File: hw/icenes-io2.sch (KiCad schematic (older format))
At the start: 35 parts, among them J4 Conn_02x31_Odd_Even, J5 Conn_02x31_Odd_Even, U4 iCE40HX8K-CT256, X2 DSC1001BI2-133.0000T

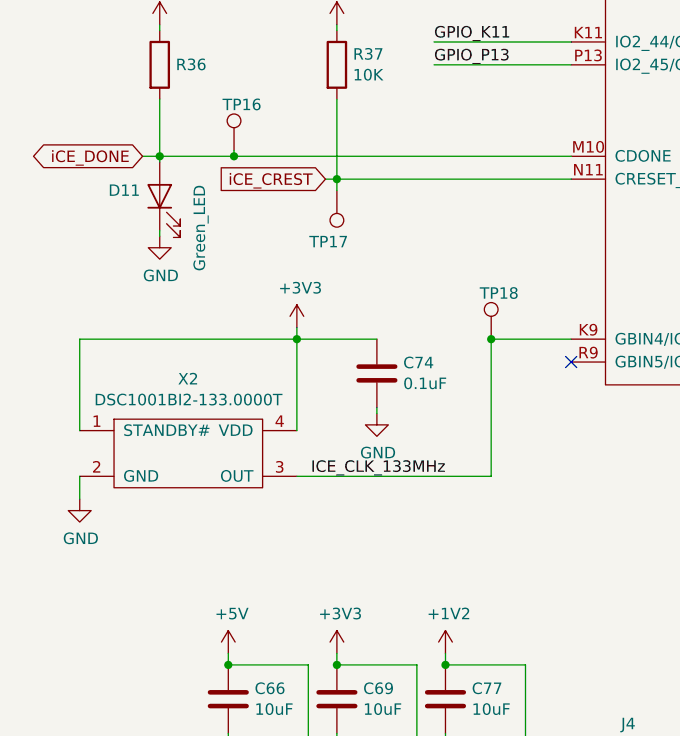
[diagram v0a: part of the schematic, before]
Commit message: Rough board layout.
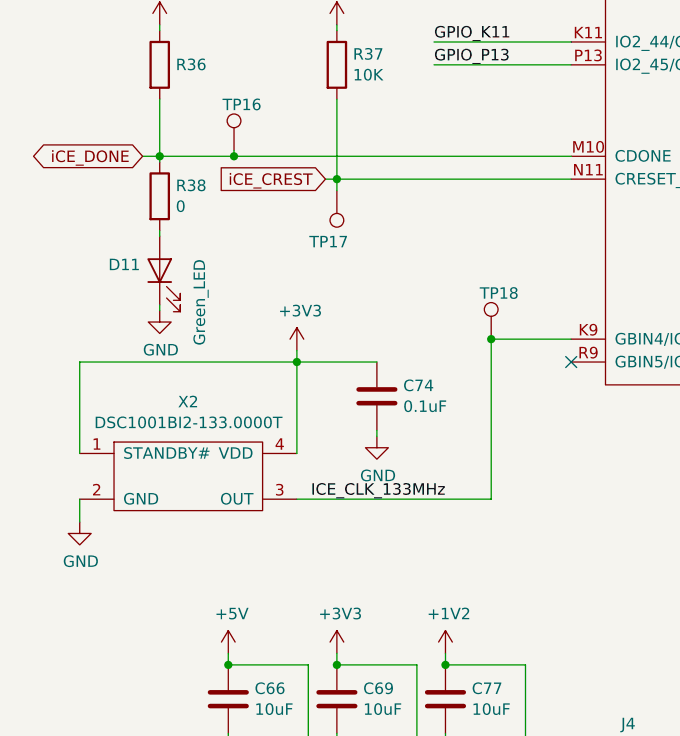
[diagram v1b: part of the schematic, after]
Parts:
- added R38: R0_0603, Resistor_SMD:R_0603_1608Metric_Pad1.05x0.95mm_HandSolder, symbol icenes-library:R0_0603
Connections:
- net iCE_DONE: now also R38.1; no longer D11.2 (A)
- new net: D11.2 (A), R38.2
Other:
- moved on the sheet: C74, D11, X2
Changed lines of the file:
@@
 L icenes-library:Green_LED D11
 U 1 1 5DA2730F
-P 1300 4775
-F 0 "D11" V 1325 5000 50  0000 R CNN
-F 1 "Green_LED" H 1350 4600 50  0000 R CNN
-F 2 "LED_SMD:LED_0805_2012Metric_Pad1.15x1.40mm_HandSolder" H 1300 4775 50  0001 C CNN
-F 3 "https://www.mouser.se/datasheet/2/216/APTD2012LCGCK-1102037.pdf" H 1300 4775 50  0001 C CNN
-F 4 "Kingbright" H 1300 4775 50  0001 C CNN "Manufacturer"
-F 5 "APTD2012LCGCK" H 1300 4775 50  0001 C CNN "Part number"
-	1    1300 4775
+P 1300 5100
+F 0 "D11" V 1325 5325 50  0000 R CNN
+F 1 "Green_LED" H 1350 4925 50  0000 R CNN
+F 2 "LED_SMD:LED_0805_2012Metric_Pad1.15x1.40mm_HandSolder" H 1300 5100 50  0001 C CNN
+F 3 "https://www.mouser.se/datasheet/2/216/APTD2012LCGCK-1102037.pdf" H 1300 5100 50  0001 C CNN
+F 4 "Kingbright" H 1300 5100 50  0001 C CNN "Manufacturer"
+F 5 "APTD2012LCGCK" H 1300 5100 50  0001 C CNN "Part number"
+	1    1300 5100
 	0    -1   -1   0
 $EndComp
@@
 L power:GND #PWR?
 U 1 1 5DA5244F
-P 1300 4950
+P 1300 5275
 AR Path="/5D1BB1FB/5DA5244F" Ref="#PWR?"  Part="1"
 AR Path="/5D1BB49B/5DA5244F" Ref="#PWR090"  Part="1"
-F 0 "#PWR090" H 1300 4700 50  0001 C CNN
-F 1 "GND" H 1305 4777 50  0000 C CNN
-F 2 "" H 1300 4950 50  0001 C CNN
-F 3 "" H 1300 4950 50  0001 C CNN
-	1    1300 4950
+F 0 "#PWR090" H 1300 5025 50  0001 C CNN
+F 1 "GND" H 1305 5102 50  0000 C CNN
+F 2 "" H 1300 5275 50  0001 C CNN
+F 3 "" H 1300 5275 50  0001 C CNN
+	1    1300 5275
 	1    0    0    -1
 $EndComp
@@
 	1300 4025 1300 4050
 Wire Wire Line
-	1300 4925 1300 4950
+	1300 5250 1300 5275
 Wire Wire Line
 	1225 4600 1300 4600
@@
 L icenes-library:C0.1uF C?
 U 1 1 5DC56E81
-P 2250 5550
+P 2250 5650
 AR Path="/5D1BAC88/5DC56E81" Ref="C?"  Part="1"
 AR Path="/5D1BB49B/5DC56E81" Ref="C74"  Part="1"
-F 0 "C74" H 2365 5596 50  0000 L CNN
-F 1 "C0.1uF" H 2100 5450 50  0001 C CNN
-F 2 "Capacitor_SMD:C_0603_1608Metric_Pad1.05x0.95mm_HandSolder" H 2250 5550 50  0001 C CNN
-F 3 "https://www.mouser.se/datasheet/2/445/885012206020-554242.pdf" H 2250 5550 50  0001 C CNN
-F 4 "0.1uF" H 2365 5505 50  0000 L CNN "Capacitance"
-F 5 "Wurth" H 2250 5550 50  0001 C CNN "Manufacturer"
-F 6 "885012206020 " H 2250 5550 50  0001 C CNN "Part number"
-	1    2250 5550
+F 0 "C74" H 2365 5696 50  0000 L CNN
+F 1 "C0.1uF" H 2100 5550 50  0001 C CNN
+F 2 "Capacitor_SMD:C_0603_1608Metric_Pad1.05x0.95mm_HandSolder" H 2250 5650 50  0001 C CNN
+F 3 "https://www.mouser.se/datasheet/2/445/885012206020-554242.pdf" H 2250 5650 50  0001 C CNN
+F 4 "0.1uF" H 2365 5605 50  0000 L CNN "Capacitance"
+F 5 "Wurth" H 2250 5650 50  0001 C CNN "Manufacturer"
+F 6 "885012206020 " H 2250 5650 50  0001 C CNN "Part number"
+	1    2250 5650
 	1    0    0    -1
 $EndComp
@@
 L power:GND #PWR?
 U 1 1 5DC56E8F
-P 2250 5725
+P 2250 5825
 AR Path="/5D1BAC88/5DC56E8F" Ref="#PWR?"  Part="1"
 AR Path="/5D1BB49B/5DC56E8F" Ref="#PWR0104"  Part="1"
-F 0 "#PWR0104" H 2250 5475 50  0001 C CNN
-F 1 "GND" H 2255 5552 50  0000 C CNN
-F 2 "" H 2250 5725 50  0001 C CNN
-F 3 "" H 2250 5725 50  0001 C CNN
-	1    2250 5725
-	1    0    0    -1
-$EndComp
-Wire Wire Line
-	1900 5400 2250 5400
-Wire Wire Line
-	1900 5400 1900 5800
-Wire Wire Line
-	1900 5350 1900 5400
-Connection ~ 1900 5400
-Wire Wire Line
-	950  5800 950  5400
-Wire Wire Line
-	950  5400 1900 5400
+F 0 "#PWR0104" H 2250 5575 50  0001 C CNN
+F 1 "GND" H 2255 5652 50  0000 C CNN
+F 2 "" H 2250 5825 50  0001 C CNN
+F 3 "" H 2250 5825 50  0001 C CNN
+	1    2250 5825
+	1    0    0    -1
+$EndComp
+Wire Wire Line
+	1900 5500 2250 5500
+Wire Wire Line
+	1900 5500 1900 5900
+Wire Wire Line
+	1900 5450 1900 5500
+Connection ~ 1900 5500
+Wire Wire Line
+	950  5900 950  5500
+Wire Wire Line
+	950  5500 1900 5500
 $Comp
 L power:GND #PWR?
 U 1 1 5DC56E9C
-P 950 6100
+P 950 6200
 AR Path="/5D1BAC88/5DC56E9C" Ref="#PWR?"  Part="1"
 AR Path="/5D1BB49B/5DC56E9C" Ref="#PWR087"  Part="1"
-F 0 "#PWR087" H 950 5850 50  0001 C CNN
-F 1 "GND" H 955 5927 50  0000 C CNN
-F 2 "" H 950 6100 50  0001 C CNN
-F 3 "" H 950 6100 50  0001 C CNN
-	1    950  6100
-	1    0    0    -1
-$EndComp
-Wire Wire Line
-	950  6000 950  6100
-Wire Wire Line
-	1900 6000 2750 6000
+F 0 "#PWR087" H 950 5950 50  0001 C CNN
+F 1 "GND" H 955 6027 50  0000 C CNN
+F 2 "" H 950 6200 50  0001 C CNN
+F 3 "" H 950 6200 50  0001 C CNN
+	1    950  6200
+	1    0    0    -1
+$EndComp
+Wire Wire Line
+	950  6100 950  6200
+Wire Wire Line
+	1900 6100 2750 6100
 $Comp
 L icenes-library:DSC1001BI2-133.0000T X2
 U 1 1 5DCE10E2
-P 1450 5700
-F 0 "X2" H 1425 5825 50  0000 C CNN
-F 1 "DSC1001BI2-133.0000T" H 1425 5734 50  0000 C CNN
-F 2 "icenes-library:MEMS_Microship_Ocillator_SMD_CDFN-4_5.0x3.2mm" H 1550 5750 50  0001 C CNN
-F 3 "https://ww1.microchip.com/downloads/en/DeviceDoc/20005529B.pdf" H 1550 5750 50  0001 C CNN
-F 4 "Microchip" H 1450 5700 50  0001 C CNN "Manufacturer"
-F 5 "DSC1001BI2-133.0000T" H 1450 5700 50  0001 C CNN "Part number"
-	1    1450 5700
-	1    0    0    -1
-$EndComp
-Wire Wire Line
-	2750 6000 2750 5400
+P 1450 5800
+F 0 "X2" H 1425 5925 50  0000 C CNN
+F 1 "DSC1001BI2-133.0000T" H 1425 5834 50  0000 C CNN
+F 2 "icenes-library:MEMS_Microship_Ocillator_SMD_CDFN-4_5.0x3.2mm" H 1550 5850 50  0001 C CNN
+F 3 "https://ww1.microchip.com/downloads/en/DeviceDoc/20005529B.pdf" H 1550 5850 50  0001 C CNN
+F 4 "Microchip" H 1450 5800 50  0001 C CNN "Manufacturer"
+F 5 "DSC1001BI2-133.0000T" H 1450 5800 50  0001 C CNN "Part number"
+	1    1450 5800
+	1    0    0    -1
+$EndComp
 Wire Wire Line
 	2750 5400 3100 5400
 NoConn ~ 3100 5500
-Text Label 2550 6000 2    50   ~ 0
+Text Label 2550 6100 2    50   ~ 0
 ICE_CLK_133MHz
 Wire Wire Line
-	2250 5725 2250 5700
+	2250 5825 2250 5800
 $Comp
 L icenes-library:TestPoint TP18
@@
 L power:+3V3 #PWR095
 U 1 1 5DDBDDE4
-P 1900 5350
-F 0 "#PWR095" H 1900 5200 50  0001 C CNN
-F 1 "+3V3" H 1915 5523 50  0000 C CNN
-F 2 "" H 1900 5350 50  0001 C CNN
-F 3 "" H 1900 5350 50  0001 C CNN
-	1    1900 5350
+P 1900 5450
+F 0 "#PWR095" H 1900 5300 50  0001 C CNN
+F 1 "+3V3" H 1915 5623 50  0000 C CNN
+F 2 "" H 1900 5450 50  0001 C CNN
+F 3 "" H 1900 5450 50  0001 C CNN
+	1    1900 5450
 	1    0    0    -1
 $EndComp
@@
 Wire Wire Line
 	2550 3000 2550 3050
+$Comp
+L icenes-library:R0_0603 R38
+U 1 1 5DCDC52E
+P 1300 4775
+F 0 "R38" V 1254 4845 50  0000 L CNN
+F 1 "R0_0603" H 1300 4675 50  0001 C CNN
+F 2 "Resistor_SMD:R_0603_1608Metric_Pad1.05x0.95mm_HandSolder" V 1300 4775 50  0001 C CNN
+F 3 "https://www.mouser.se/datasheet/2/447/PYu-RC_Group_51_RoHS_L_10-1527934.pdf" V 1300 4775 50  0001 C CNN
+F 4 "0" V 1345 4845 50  0000 L CNN "Resistance"
+F 5 "Yageo" H 1300 4775 50  0001 C CNN "Manufacturer"
+F 6 "RC0603FR-070RL" H 1300 4775 50  0001 C CNN "Part number"
+	1    1300 4775
+	0    1    1    0
+$EndComp
+Wire Wire Line
+	1300 4925 1300 4950
+Wire Wire Line
+	2750 5400 2750 6100
 $EndSCHEMATC
